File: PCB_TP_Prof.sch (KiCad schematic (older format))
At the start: 18 parts, among them J1 Conn_01x16_Female, J2 Conn_01x12_Female, J3 Conn_01x16_Female, J4 Conn_01x01_Male, J5 Conn_01x01_Male, J6 Conn_01x01_Male

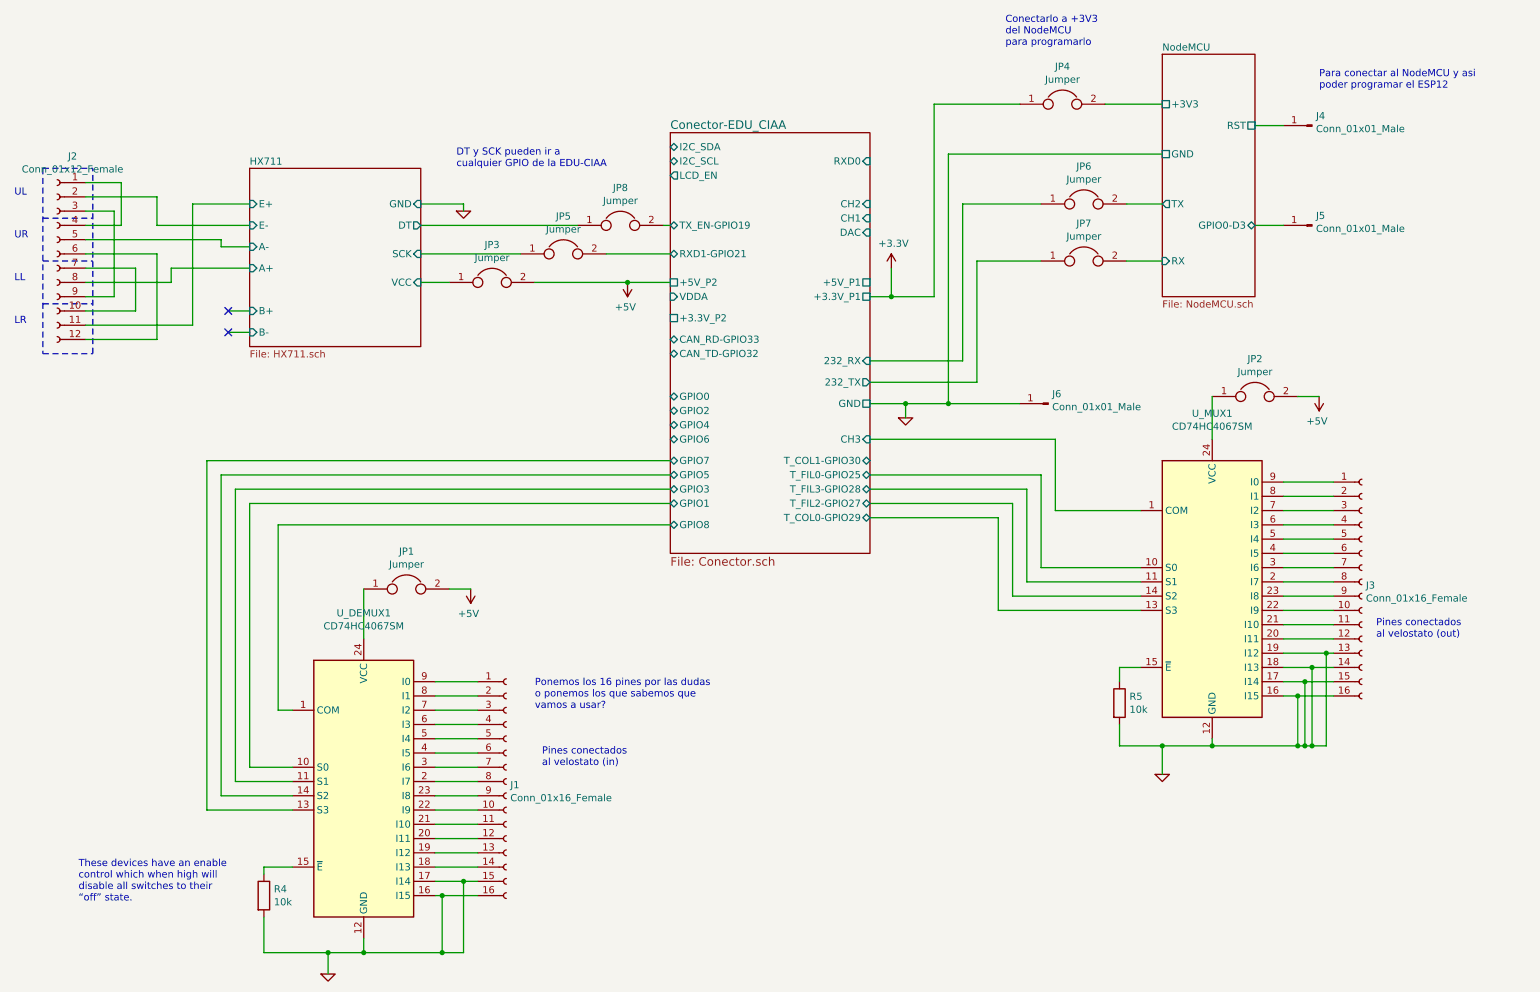
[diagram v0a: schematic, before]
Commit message: Update files + gerbers
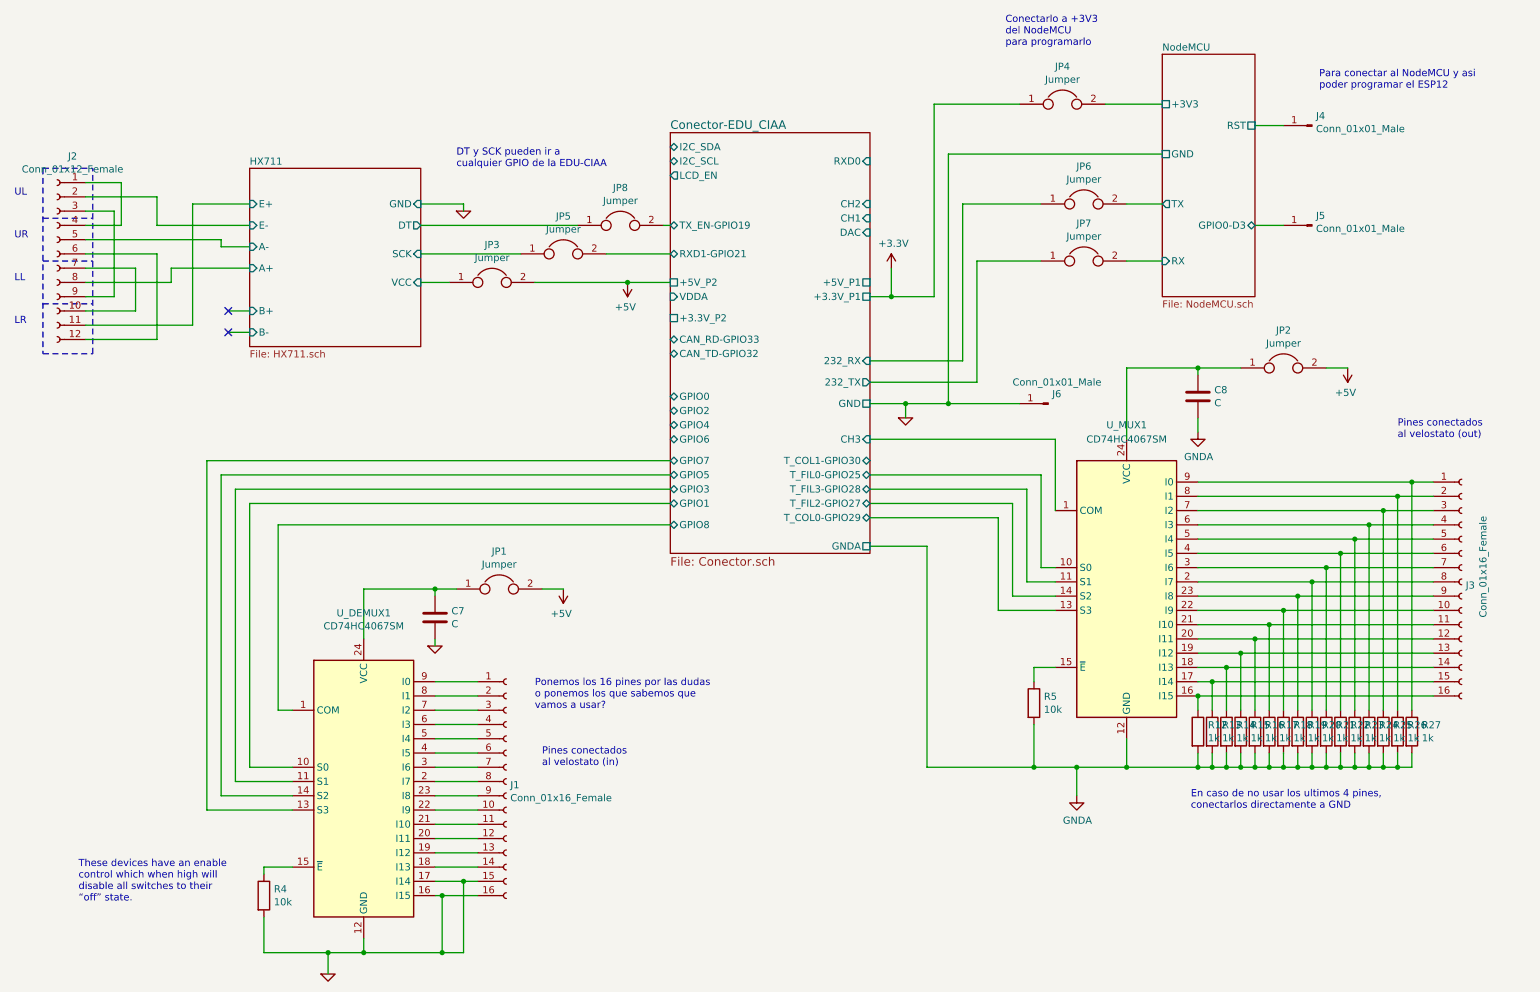
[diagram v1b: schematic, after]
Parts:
- added C7, C8: C, Capacitor_SMD:C_1206_3216Metric_Pad1.33x1.80mm_HandSolder, symbol Device:C
- added R12, R13, R14, R15, R16, R17, R18, R19, R20, R21, R22, R23, R24, R25, R26, R27: 1k, Resistor_SMD:R_1206_3216Metric, symbol Device:R
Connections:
- net GND: now also C7.2; no longer J3.13 (Pin_13), J3.14 (Pin_14), J3.15 (Pin_15), J3.16 (Pin_16), R5.2, U_MUX1.12 (GND), U_MUX1.16 (I15), U_MUX1.17 (I14), U_MUX1.18 (I13), U_MUX1.19 (I12)
- net at JP1.1, U_DEMUX1.24 (VCC): now also C7.1
- net at JP2.1, U_MUX1.24 (VCC): now also C8.2
- net at J3.1 (Pin_1), U_MUX1.9 (I0): now also R27.1
- net at J3.10 (Pin_10), U_MUX1.22 (I9): now also R18.1
- net at J3.11 (Pin_11), U_MUX1.21 (I10): now also R17.1
- net at J3.12 (Pin_12), U_MUX1.20 (I11): now also R16.1
- net at J3.2 (Pin_2), U_MUX1.8 (I1): now also R26.1
- net at J3.3 (Pin_3), U_MUX1.7 (I2): now also R25.1
- net at J3.4 (Pin_4), U_MUX1.6 (I3): now also R24.1
- net at J3.5 (Pin_5), U_MUX1.5 (I4): now also R23.1
- net at J3.6 (Pin_6), U_MUX1.4 (I5): now also R22.1
- net at J3.7 (Pin_7), U_MUX1.3 (I6): now also R21.1
- net at J3.8 (Pin_8), U_MUX1.2 (I7): now also R20.1
- net at J3.9 (Pin_9), U_MUX1.23 (I8): now also R19.1
- new net: J3.13 (Pin_13), R15.1, U_MUX1.19 (I12)
- new net: J3.14 (Pin_14), R14.1, U_MUX1.18 (I13)
- new net: J3.15 (Pin_15), R13.1, U_MUX1.17 (I14)
- new net: J3.16 (Pin_16), R12.1, U_MUX1.16 (I15)
- new net GNDA: C8.1, R12.2, R13.2, R14.2, R15.2, R16.2, R17.2, R18.2, R19.2, R20.2, R21.2, R22.2, R23.2, R24.2, R25.2, R26.2, R27.2, R5.2, U_MUX1.12 (GND)
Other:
- note added: "En caso de no usar los ultimos 4 pines, \nconectarlos directamente a GND\n"
- moved on the sheet: J3, JP1, JP2, R5, U_MUX1
